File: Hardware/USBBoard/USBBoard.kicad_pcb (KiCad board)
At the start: 2 copper layers, 27.9 x 38.1 mm, 48 parts, among them J1 USB_C_Receptacle_USB2.0, J2 POWERBOARD, Q1 BS170F, Q2 BS170F, Q3 BC846, Q4 BC846, Q5 AO3401A, Q6 2N7002, U1 CH340C, U2 FS8205A, U3 XC6203, U4 TC4056A, U6 DW01-P, U7 XC6203

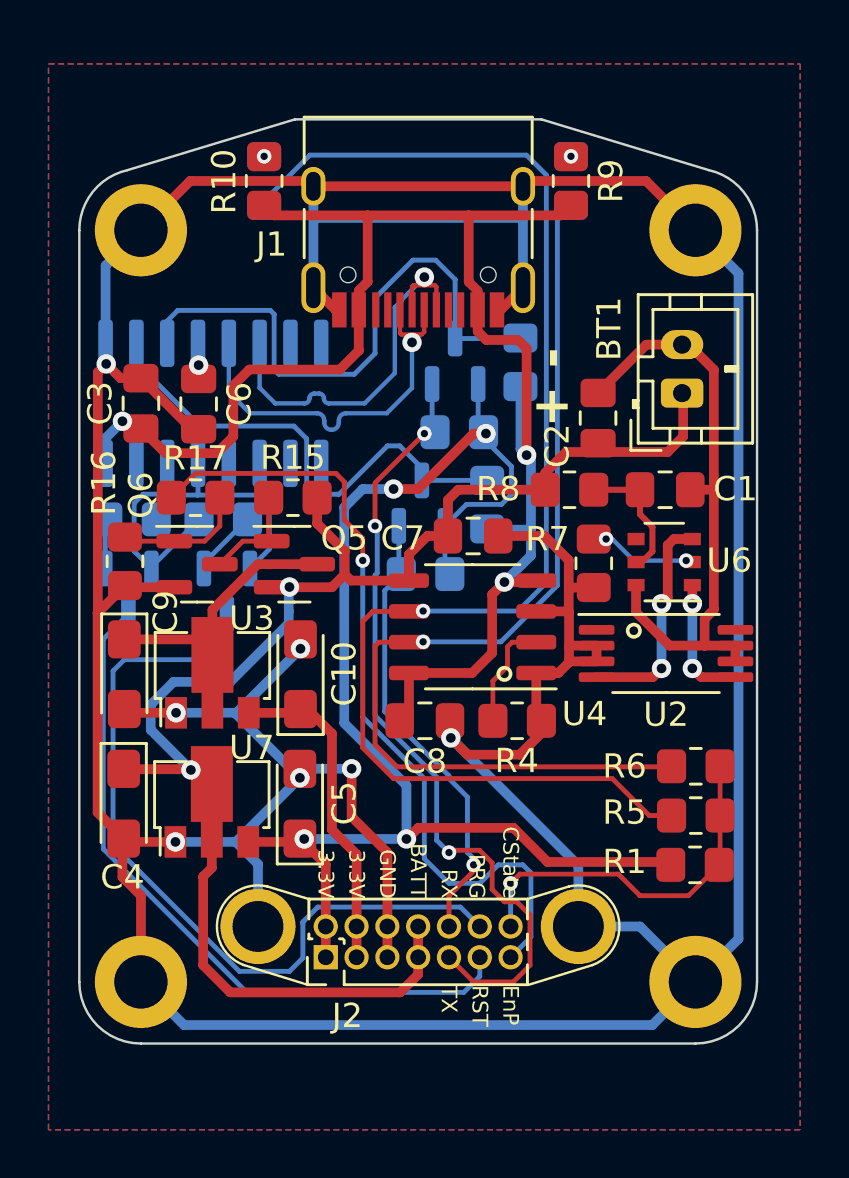
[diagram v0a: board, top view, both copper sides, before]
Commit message: USBBoard tweaks
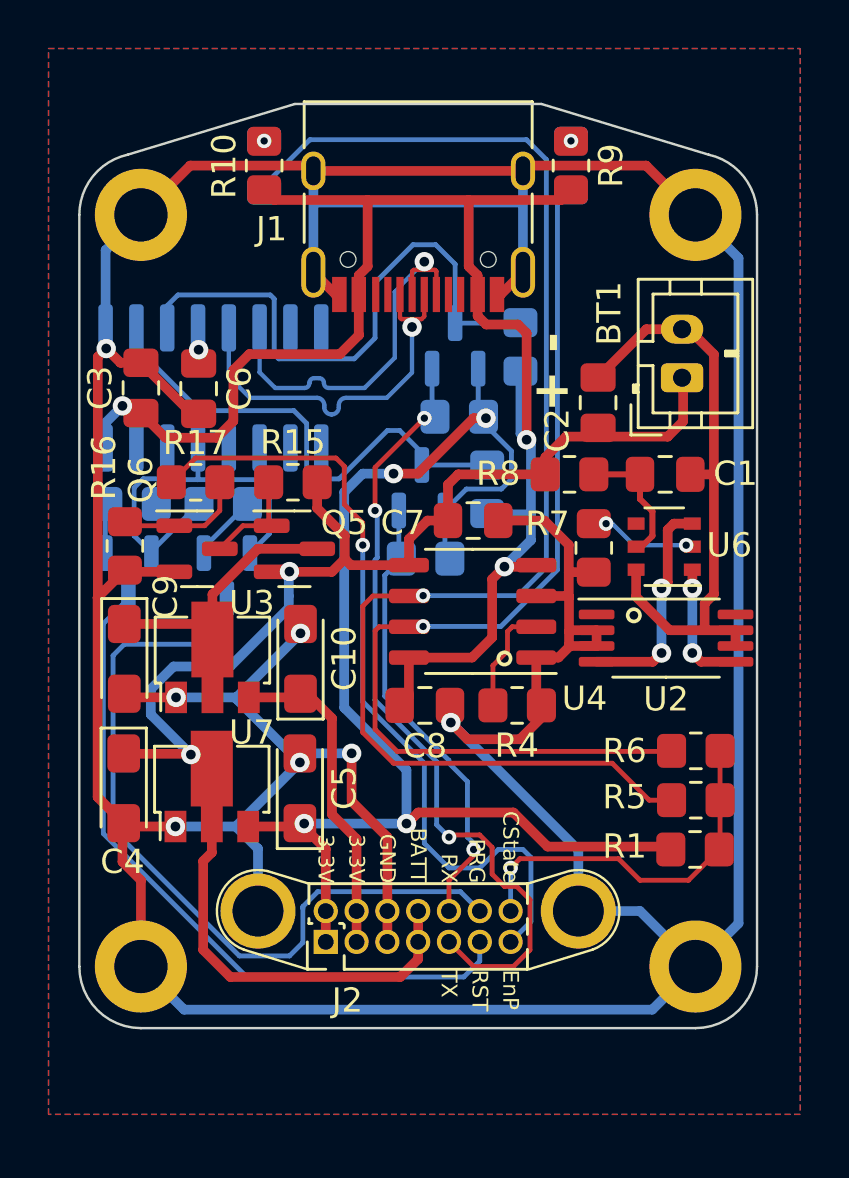
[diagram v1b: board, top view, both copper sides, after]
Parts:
- moved BT1 0.64 mm to (10.9, -22.6)
- moved C1 0.64 mm to (10.2, -18.6)
- moved C2 0.64 mm to (7.42, -21.6)
- moved J1 0.64 mm to (0.00, -30.1)
- moved Q2 0.64 mm to (1.52, -23.9)
- moved R16 0.64 mm to (-12.1, -15.7)
- moved R8 0.64 mm to (6.24, -18.6)
- moved U7 0.64 mm to (-8.51, -6.07)
- moved H3 0.64 mm to (11.4, 1.65)
- moved H4 0.64 mm to (-11.4, 1.65)
- moved J2 0.64 mm to (0.00, 0.00)
- moved C10 0.63 mm to (-4.85, -11.0)
- moved C4 0.63 mm to (-12.1, -5.70)
- moved C5 0.63 mm to (-4.88, -5.70)
- moved C8 0.63 mm to (0.28, -9.11)
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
